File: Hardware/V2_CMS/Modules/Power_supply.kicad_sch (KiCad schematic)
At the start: 33 parts, among them J12 GND, J13 GND, J14 GND, U10 L7805, U11 AMS1117-3.3, U12 LM317_TO-220

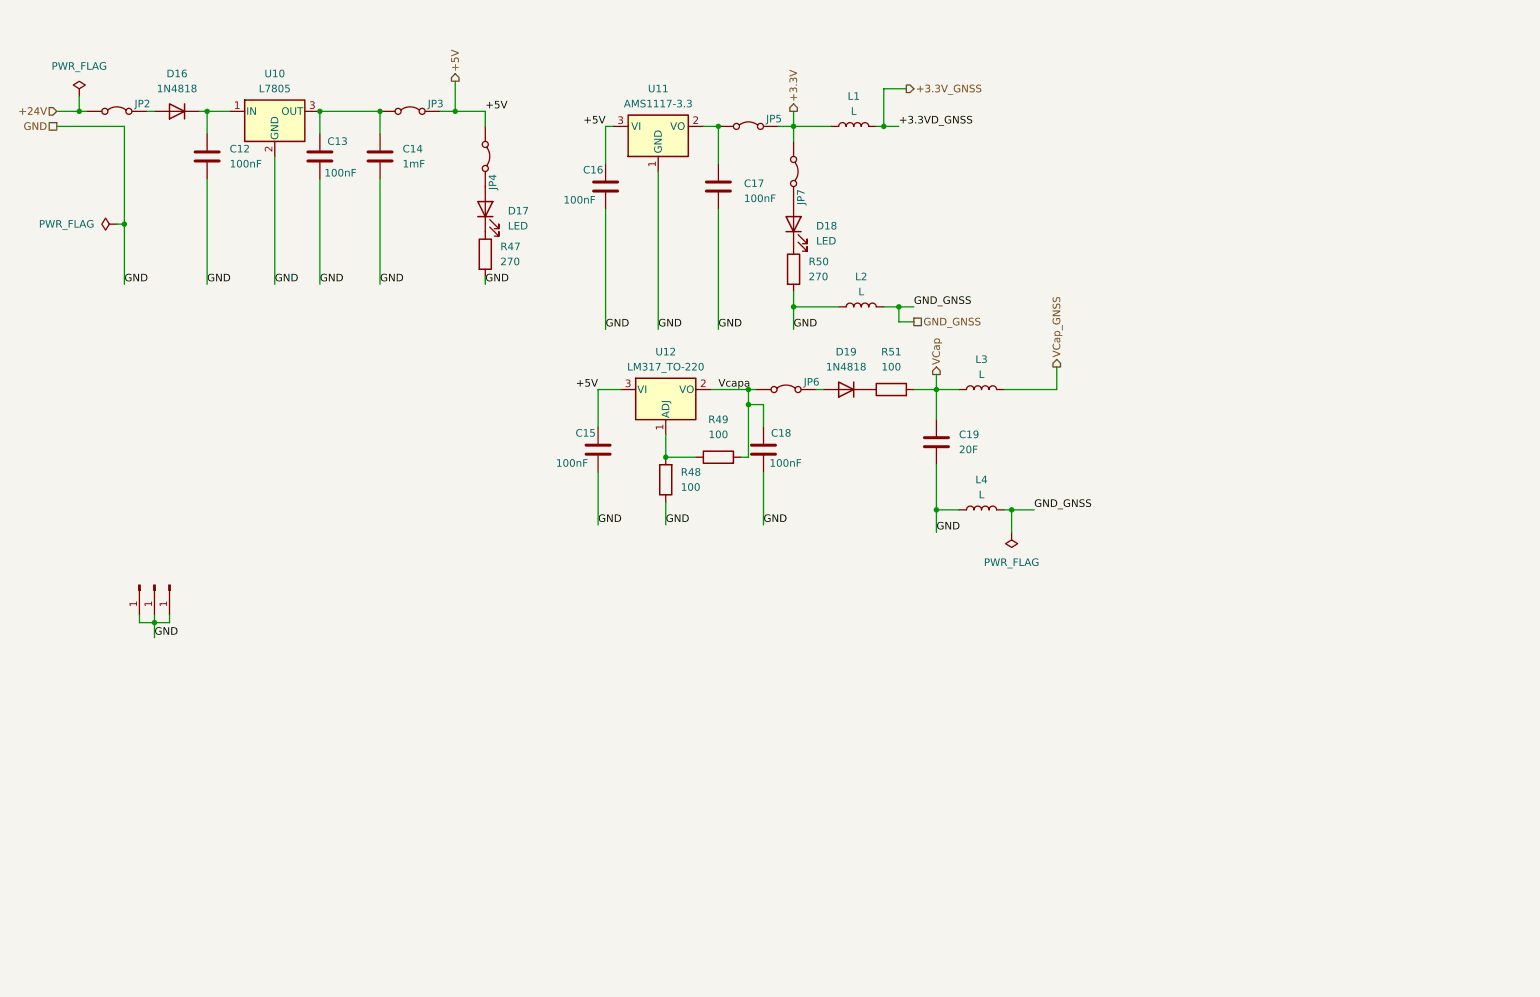
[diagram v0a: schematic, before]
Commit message: update of directory
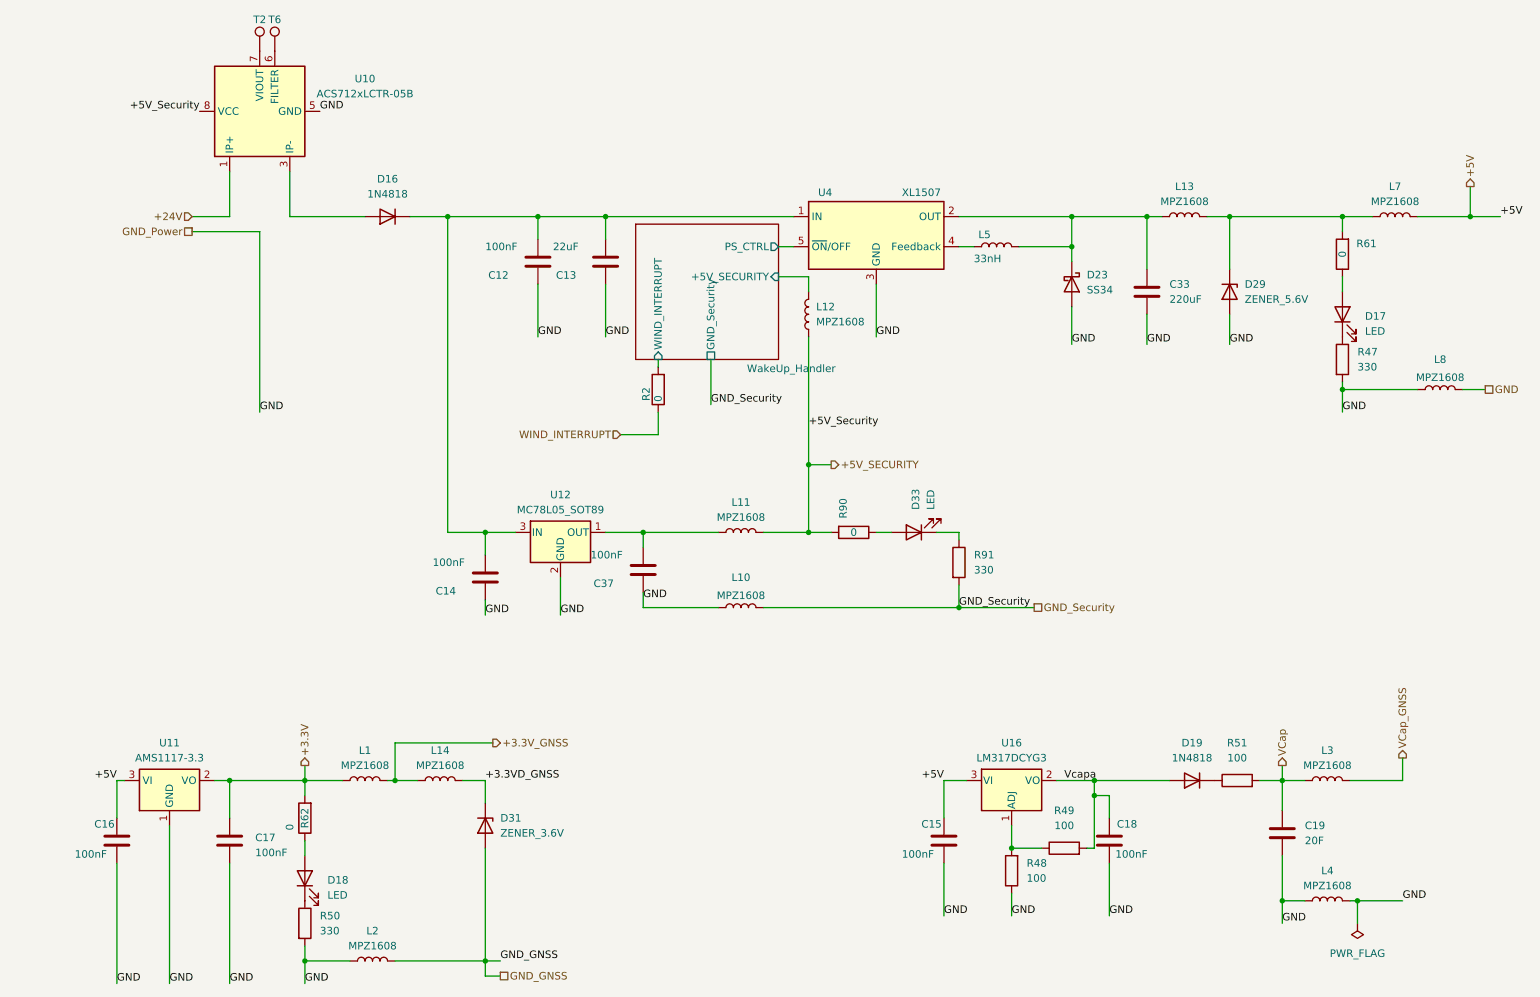
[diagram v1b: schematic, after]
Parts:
- removed J12, J13, J14: GND, Connector_PinHeader_2.54mm:PinHeader_1x01_P2.54mm_Vertical, symbol Connector:Conn_01x01_Pin
- removed JP2, JP3, JP4, JP5, JP6, JP7: Jumper, Connector_PinHeader_2.54mm:PinHeader_1x02_P2.54mm_Vertical, symbol Jumper:Jumper_2_Bridged
- removed U10: L7805, Package_TO_SOT_THT:TO-220-3_Vertical, symbol Regulator_Linear:L7805
- removed U12: LM317_TO-220, Package_TO_SOT_THT:TO-220-3_Vertical, symbol Regulator_Linear:LM317_TO-220
- added C33: 220uF, Capacitor_SMD:CP_Elec_6.3x7.7, symbol Device:C
- added C37: 100nF, Capacitor_SMD:C_0603_1608Metric, symbol Device:C
- added D23: SS34, Diode_SMD:D_SMA, symbol Diode:SS34
- added D29: ZENER_5.6V, Diode_SMD:D_MiniMELF, symbol Device:D_Zener
- added D31: ZENER_3.6V, Diode_SMD:D_MiniMELF, symbol Device:D_Zener
- added D33: LED, LED_SMD:LED_0603_1608Metric, symbol Device:LED
- added L10, L11, L12, L13, L14, L7, L8: MPZ1608, Inductor_SMD:L_0603_1608Metric, symbol Device:L
- added L5: 33nH, Inductor_SMD:L_Wuerth_HCI-5040, symbol Device:L
- added R2, R61, R62, R90: 0, Resistor_SMD:R_0603_1608Metric, symbol Device:R
- added R91: 330, Resistor_SMD:R_0603_1608Metric, symbol Device:R
- added T2, T6: TP, TestPoint:TestPoint_Pad_D1.0mm, symbol Connector:TestPoint
- added U10: ACS712xLCTR-05B, Package_SO:SOIC-8_3.9x4.9mm_P1.27mm, symbol Sensor_Current:ACS712xLCTR-05B
- added U12: MC78L05_SOT89, Package_TO_SOT_SMD:SOT-89-3, symbol Regulator_Linear:MC78L05_SOT89
- added U16: LM317DCYG3, Package_TO_SOT_SMD:SOT-223-3_TabPin2, symbol Regulator_Linear:LM317_SOT-223
- added U4: XL1507, Package_TO_SOT_SMD:TO-252-5_TabPin3, symbol Power_Management:BTS443P
- C13: value 100nF -> 22uF
- C14: value 1mF -> 100nF
- D16: footprint Diode_SMD:D_0603_1608Metric -> Diode_SMD:D_SOD-323
- D19: footprint Diode_THT:D_DO-41_SOD81_P7.62mm_Horizontal -> Diode_SMD:D_SOD-323
- L1, L2, L3, L4: value L -> MPZ1608
- R47, R50: value 270 -> 330
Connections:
- net +24V: now also U10.1 (IP+), U10.2 (IP+)
- net +3.3V: now also C17.1, U11.2 (VO), R62.2
- net +3.3V_GNSS: now also L14.1
- net +5V: now also L7.2, U16.3 (VI)
- net GND: now also L4.2, C33.2, C37.2, D23.2 (A), D29.2 (A), L10.1, L8.1, L8.2, U10.5 (GND), U12.2 (GND), U4.3 (GND)
- net GND_GNSS: now also D31.2 (A); no longer L4.2
- net Vcapa: now also D19.2 (A), U16.2 (VO)
- net at C12.1, D16.1 (K): now also C13.1, C14.1, U12.3 (IN), U4.1 (IN)
- net at D16.2 (A): now also U10.3 (IP-), U10.4 (IP-)
- net at R48.2, R49.1: now also U16.1 (ADJ)
- net at D17.2 (A): now also R61.1
- net at D18.2 (A): now also R62.1
- new net: C37.1, L11.1, U12.1 (OUT)
- new net: D29.1 (K), L13.2, L7.1, R61.2
- new net: C33.1, D23.1 (K), L13.1, L5.2, U4.2 (OUT)
- new net: L5.1, U4.4 (Feedback)
- new net: D33.2 (A), R90.1
- new net: T2.1, U10.7 (VIOUT)
- new net: T6.1, U10.6 (FILTER)
- new net: D33.1 (K), R91.1
- new net +3.3VD_GNSS: D31.1 (K), L14.2
- new net +5V_SECURITY: L11.2, L12.1, R90.2, U10.8 (VCC)
- new net GND_Security: L10.2, R91.2
- new net WIND_INTERRUPT: R2.1
- new net WakeUp_Handler/+5V_SECURITY: L12.2
- new net WakeUp_Handler/PS_CTRL: U4.5 (~{ON}/OFF)
- new net WakeUp_Handler/WIND_INTERRUPT: R2.2
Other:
- added sheet WakeUp_Handler (WakeUp_Handler.kicad_sch)
- moved on the sheet: C12, C15, C16, C17, C18, C19, D16, D17, D18, D19, L1, L2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
